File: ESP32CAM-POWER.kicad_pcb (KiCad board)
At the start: 2 copper layers, 33.5 x 39 mm, 18 parts, among them J1 Conn_01x02_Female, J2 Conn_01x06_Male, U1 D-SUN-MP1584EN, U2 ESP32-CAM

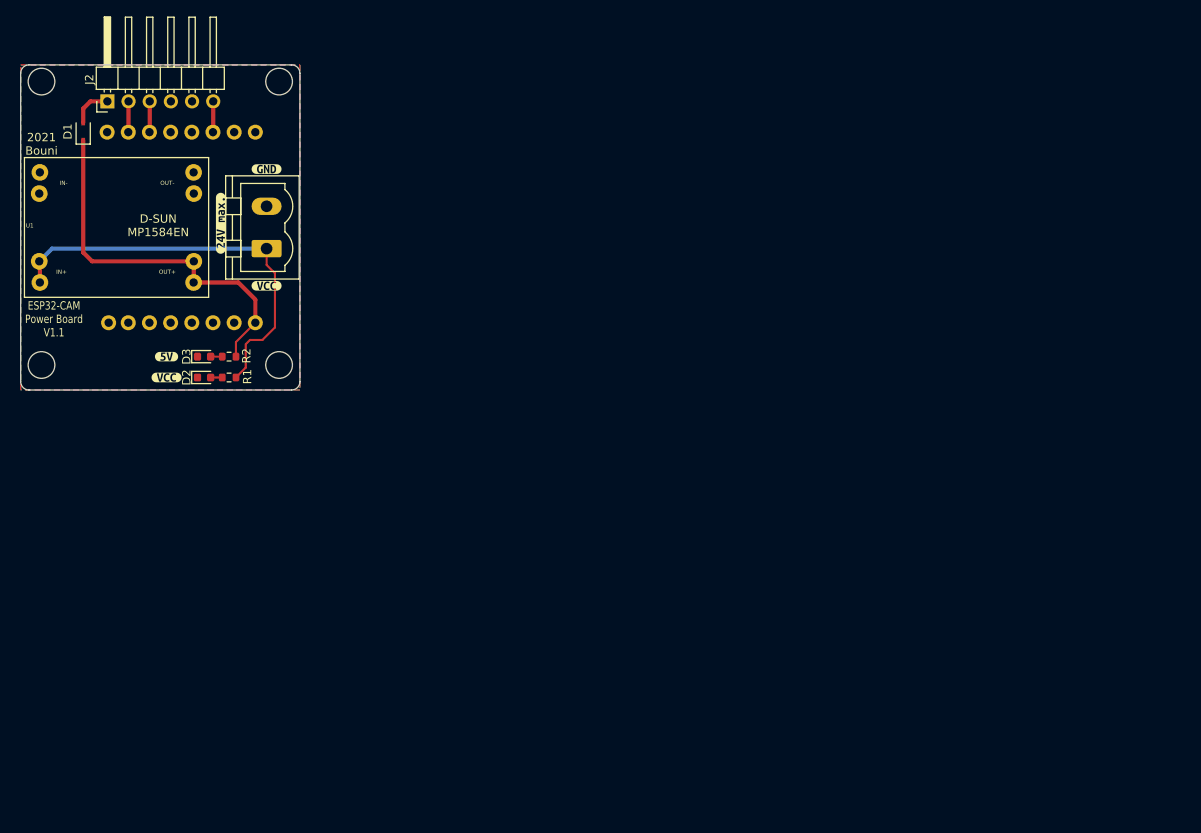
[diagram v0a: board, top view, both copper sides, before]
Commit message: some chages for V1.3
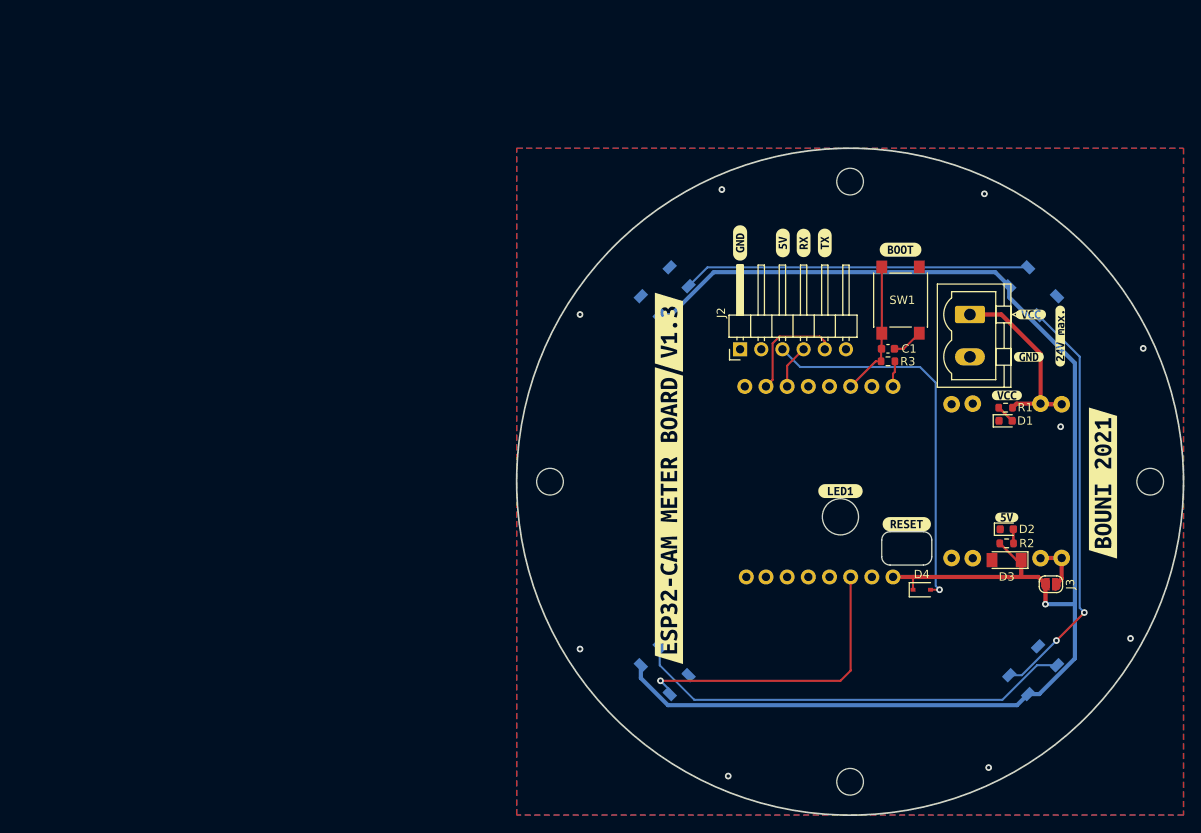
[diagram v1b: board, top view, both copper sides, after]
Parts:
- added C1: 100nF, Capacitor_SMD:C_0603_1608Metric, F.Cu at (154.5, 64.1)
- added D3: BZV55C5V1, Diode_SMD:D_MiniMELF, F.Cu at (168.8, 89.4)
- added D5: WS2812B, LED_SMD:LED_WS2812B_PLCC4_5.0x5.0mm_P3.2mm, B.Cu at (127.8, 102.6)
- added D6: WS2812B, LED_SMD:LED_WS2812B_PLCC4_5.0x5.0mm_P3.2mm, B.Cu at (172.0, 102.6)
- added D7: WS2812B, LED_SMD:LED_WS2812B_PLCC4_5.0x5.0mm_P3.2mm, B.Cu at (172.0, 57.1)
- added D8: WS2812B, LED_SMD:LED_WS2812B_PLCC4_5.0x5.0mm_P3.2mm, B.Cu at (127.8, 57.1)
- added J3: Conn_01x02_Male, Jumper:SolderJumper-2_P1.3mm_Open_RoundedPad1.0x1.5mm, F.Cu at (174.1, 92.3)
- added R3: 10k, Resistor_SMD:R_0603_1608Metric, F.Cu at (154.5, 65.6)
- added SW1: BOOT, Button_Switch_SMD:SW_Push_1P1T_NO_6x6mm_H9.5mm, F.Cu at (156.1, 58.2)
- added kibuzzard-61893861: G***, kibuzzard-61893861, F.Cu at (180.3, 80.2)
- added kibuzzard-61893876: G***, kibuzzard-61893876, F.Cu at (141.9, 51.4)
- added kibuzzard-61893880: G***, kibuzzard-61893880, F.Cu at (147.0, 51.4)
- added kibuzzard-61893893: G***, kibuzzard-61893893, F.Cu at (144.4, 51.4)
- added kibuzzard-6189389B: G***, kibuzzard-6189389B, F.Cu at (136.8, 51.4)
- added kibuzzard-61893A2D: G***, kibuzzard-61893A2D, F.Cu at (156.8, 85.1)
- added kibuzzard-61893D50: G***, kibuzzard-61893D50, F.Cu at (128.3, 84.1)
- added kibuzzard-61893E19: G***, kibuzzard-61893E19, F.Cu at (156.1, 52.2)
- added kibuzzard-619E5A56: G***, kibuzzard-619E5A56, F.Cu at (148.8, 81.1)
- added kibuzzard-619E5D40: G***, kibuzzard-619E5D40, F.Cu at (128.3, 62.1)
- U1: moved to B.Cu
- moved H4 141.4 mm to (186.0, 80.0)
- moved D4 114.6 mm to (158.6, 93.0), turned to 0 degrees
- moved U1 111.0 mm to (168.8, 79.9), turned to -90 degrees
- moved kibuzzard-611BC01E 102.6 mm to (168.8, 84.3)
- moved kibuzzard-611BC02E 101.6 mm to (175.2, 62.5)
- moved kibuzzard-611BC015 100.8 mm to (168.8, 69.6)
- moved D2 98.5 mm to (168.8, 85.7)
- moved D1 96.3 mm to (168.7, 72.7)
- moved R2 95.9 mm to (168.8, 87.4), turned to 0 degrees
- moved kibuzzard-611BBF3F 94.2 mm to (171.4, 65.0)
- moved R1 93.2 mm to (168.7, 71.1)
- moved kibuzzard-611BBF47 91.8 mm to (171.7, 59.9)
- moved H1 84.8 mm to (150.0, 116.0)
- moved J1 84.7 mm to (164.4, 59.9), turned to -90 degrees
- moved U2 82.4 mm to (140.0, 80.0)
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- renumbered D2 to D1, D3 to D2, D1 to D4
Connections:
- D4 pad 2: Net-(D1-Pad2) (its old number) -> Net-(J2-Pad3)
- J2 pad 1: Net-(D1-Pad2) (its old number) -> GND
- J2 pad 2: TX -> unconnected-(J2-Pad2)
- J2 pad 3: RX -> Net-(J2-Pad3)
- J2 pad 4: GND -> RX
- J2 pad 5: GND -> TX
- J2 pad 6: BOOT -> unconnected-(J2-Pad6)
- U1 pad 7: +5V -> Net-(U1-Pad7)
- U1 pad 8: +5V -> Net-(U1-Pad7)
- U2 pad 10: (no net) -> unconnected-(U2-Pad10)
- U2 pad 13: (no net) -> unconnected-(U2-Pad13)
- U2 pad 3: (no net) -> LED
- U2 pad 4: (no net) -> unconnected-(U2-Pad4)
- U2 pad 5: (no net) -> unconnected-(U2-Pad5)
- U2 pad 6: (no net) -> unconnected-(U2-Pad6)
- U2 pad 7: (no net) -> unconnected-(U2-Pad7)
- U2 pad 8: (no net) -> unconnected-(U2-Pad8)
- U2 pad 9: (no net) -> +3V3
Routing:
- net +5V: track 45.8 -> 181.6 mm, vias 0 -> 1
- net Net-(D5-Pad2): track 0.00 -> 53.4 mm
- net Net-(D6-Pad2): track 0.00 -> 50.1 mm, vias 0 -> 2
- net Net-(J2-Pad3): track 0.00 -> 46.2 mm, vias 0 -> 1
- net Net-(D7-Pad2): track 0.00 -> 41.7 mm
- net LED: track 0.00 -> 36.6 mm, vias 0 -> 1
- net VCC: track 49.2 -> 22.5 mm
- net BOOT: track 3.71 -> 16.3 mm
- net TX: track 3.71 -> 13.3 mm
- net Net-(U1-Pad7): track 0.00 -> 5.97 mm
- net Net-(D1-Pad2) (its old number): track 4.96 -> 0.00 mm
- net GND: track 0.00 -> 3.76 mm, vias 0 -> 9
- net +3V3: track 0.00 -> 3.18 mm
- net RX: track 3.71 -> 5.27 mm
- net Net-(D1-Pad2): track 1.39 -> 2.27 mm
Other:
- board size 33.5 x 39 mm -> 80 x 80 mm
- board text removed: "2021 Bouni"
- board text removed: "ESP32-CAM Power Board V1.1"
- board text removed: "JLCJLCJLCJLC"
